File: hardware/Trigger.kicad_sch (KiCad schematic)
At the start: 8 parts, among them U6 MCP47FEB02A0T-E/ST, U7 Opamp_Dual

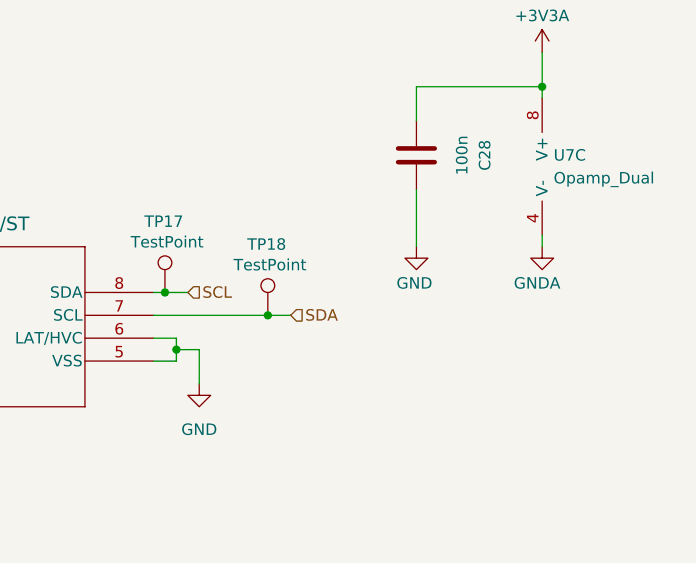
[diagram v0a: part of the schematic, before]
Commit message: feat(hardware): Finish component layout
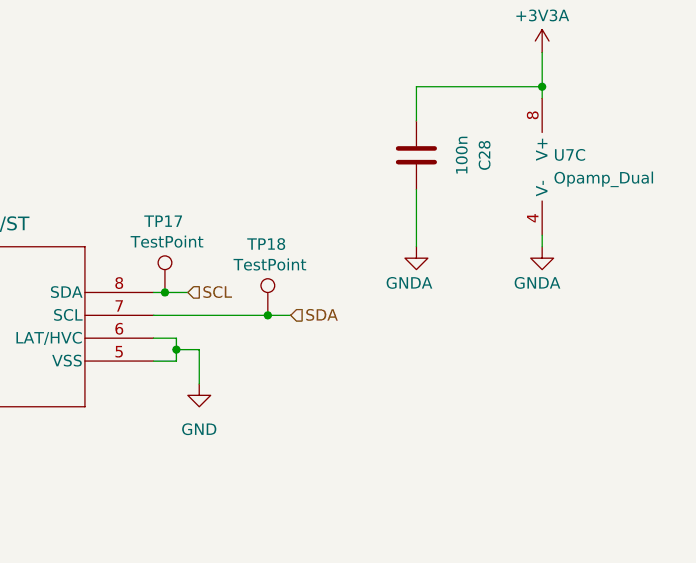
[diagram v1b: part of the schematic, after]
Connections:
- net GND: no longer C28.2
- net GNDA: now also C28.2
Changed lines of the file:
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@@
 			)
 		)
-		(property "Value" "GND"
+		(property "Value" "GNDA"
 			(at 142.748 82.804 0)
 			(effects

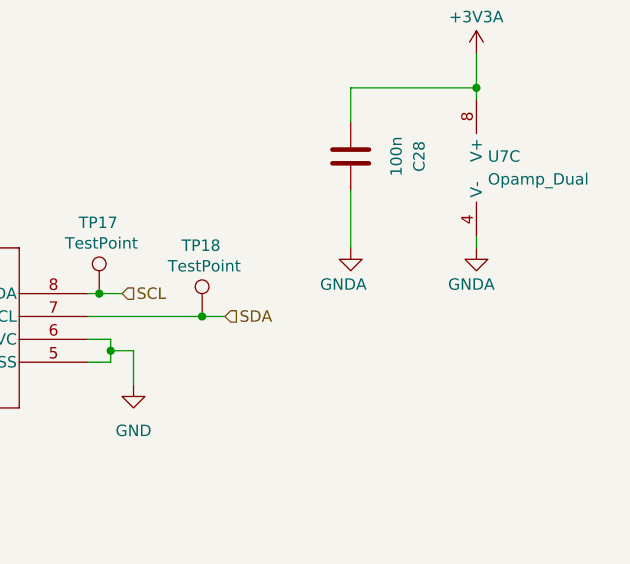
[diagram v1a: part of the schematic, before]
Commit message: feat(hardware): updted design rules
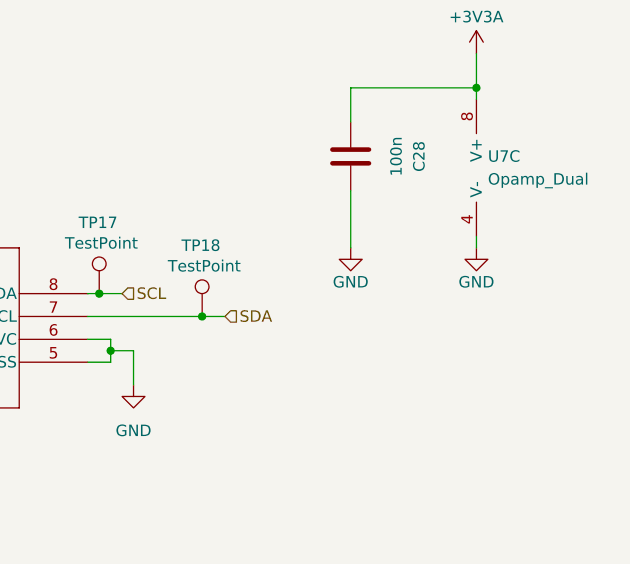
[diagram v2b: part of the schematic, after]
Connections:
- net GNDA is gone; now on net GND: C28.2, U7.4 (V-)
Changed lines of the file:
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@@
 			)
 		)
-		(property "Value" "GNDA"
-			(at 156.972 82.804 0)
-			(effects
-				(font
-					(size 1.27 1.27)
-				)
-				(justify right)
+		(property "Value" "GND"
+			(at 154.94 82.55 0)
+			(effects
+				(font
+					(size 1.27 1.27)
+				)
 			)
 		)
@@
 			)
 		)
-		(property "Value" "GNDA"
-			(at 142.748 82.804 0)
-			(effects
-				(font
-					(size 1.27 1.27)
-				)
-				(justify right)
-			)
-		)
+		(property "Value" "GND"
+			(at 140.97 82.55 0)
+			(effects
+				(font
+					(size 1.27 1.27)
+				)
+			)
+		)
